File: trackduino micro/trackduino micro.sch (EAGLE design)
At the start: 28 parts, among them IC2 74AHC1G125DBV, SW1 SPST_TACT-KMR2, U1 ATMEGA168MLF, Y1 16MHZ

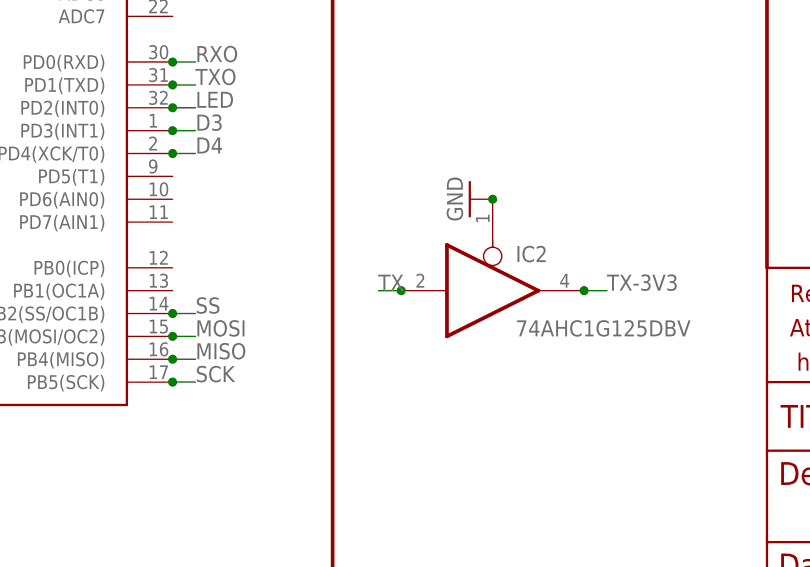
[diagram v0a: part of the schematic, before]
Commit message: re-routed micro board
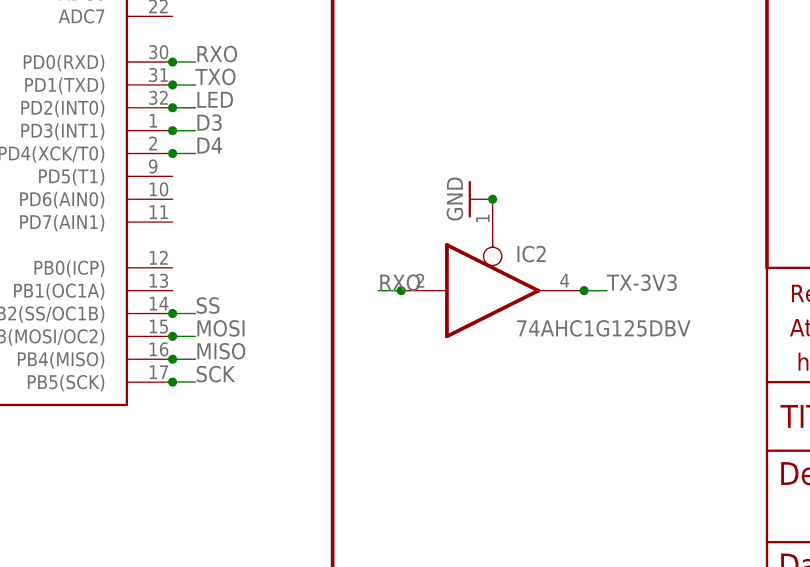
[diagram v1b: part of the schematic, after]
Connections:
- net RXO: now also IC2A.I
- net TX: no longer IC2A.I
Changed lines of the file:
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@@
 <net name="TX" class="0">
-<segment>
-<pinref part="IC2" gate="A" pin="I"/>
-<wire x1="106.68" y1="33.02" x2="104.14" y2="33.02" width="0.1524" layer="91"/>
-<label x="104.14" y="33.02" size="1.778" layer="95"/>
-<junction x="106.68" y="33.02"/>
-</segment>
 <segment>
 <wire x1="220.98" y1="134.62" x2="223.52" y2="134.62" width="0.1524" layer="91"/>
@@
 <junction x="203.2" y="50.8"/>
 </segment>
-</net>
+<segment>
+<pinref part="IC2" gate="A" pin="I"/>
+<wire x1="106.68" y1="33.02" x2="104.14" y2="33.02" width="0.1524" layer="91"/>
+<label x="104.14" y="33.02" size="1.778" layer="95"/>
+<junction x="106.68" y="33.02"/>
+</segment>
+</net>
